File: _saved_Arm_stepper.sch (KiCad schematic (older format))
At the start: 126 parts, among them IC1 L6208D, IC2 L6208D, J1 12V_CONN, J10 ENCODER1, J11 ENCODER2, J2 M1_CONN, J3 M1_CONN, J4 Conn_01x06_Male, J5 I2C_CONN, J8 Conn_01x04_Female, J9 USB_B_Mini, M2 Fan, Q2 2N2219, SW1 SW_Push_Dual, SW2 endstop4, SW3 endstop1, SW4 endstop3, SW5 endstop2, U1 ISO1050-00_isolation, U2 USBLC6-2SC6, U3 STM32F446RETx, U4 LM1117-3.3, U5 LM1117-5, Y1 8Mhz

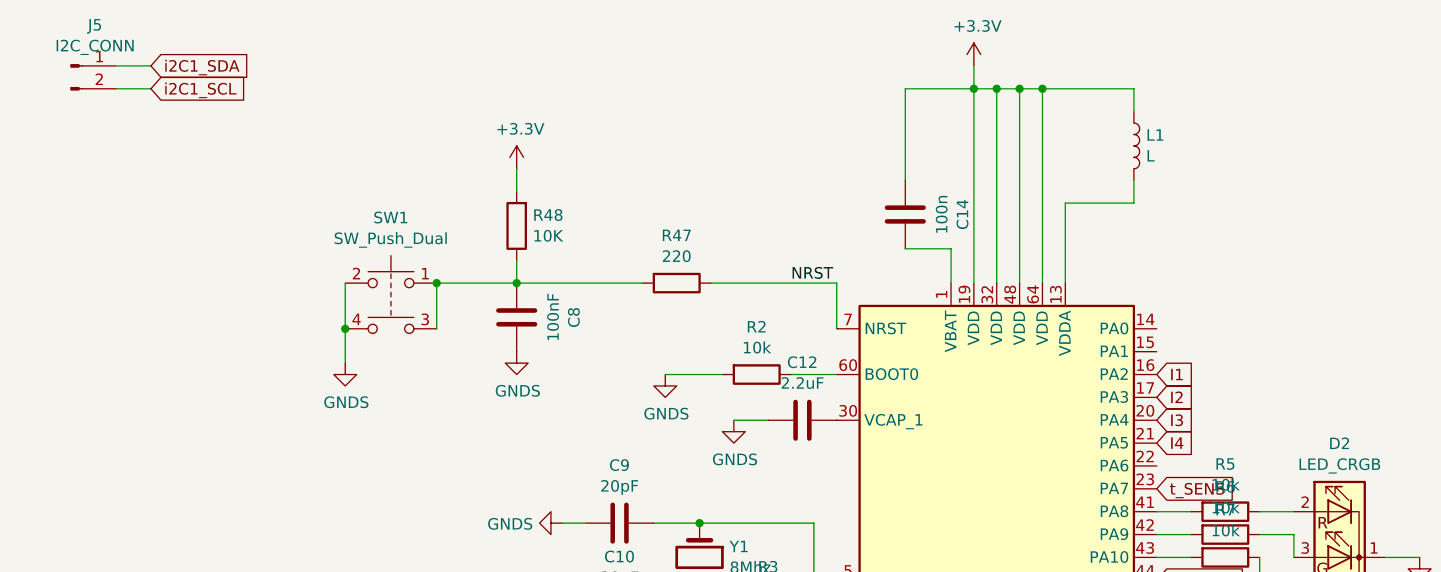
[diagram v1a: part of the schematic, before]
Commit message: finish4
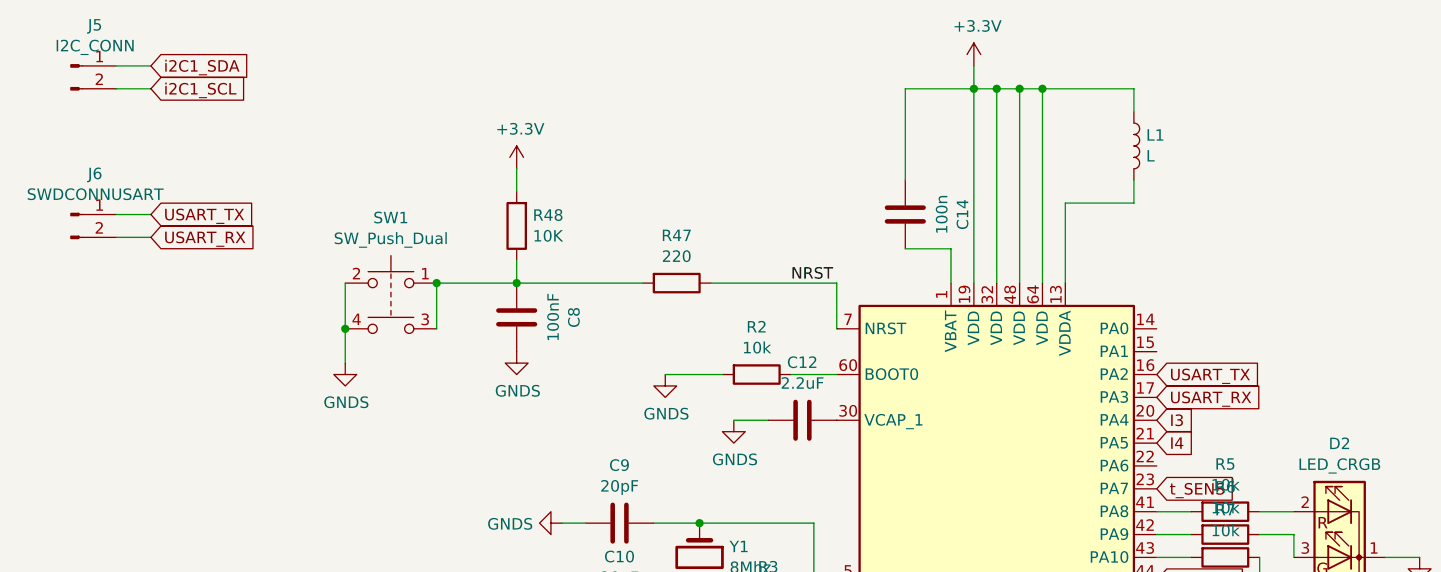
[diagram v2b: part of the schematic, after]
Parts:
- added J6: SWDCONNUSART, TerminalBlock_Phoenix:TerminalBlock_Phoenix_MPT-0,5-4-2.54_1x04_P2.54mm_Horizontal, symbol Connector:Conn_01x02_Male
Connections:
- net I1 renamed USART_TX
- net USART_TX: now also J6.1 (Pin_1)
- net I2 renamed USART_RX
- net USART_RX: now also J6.2 (Pin_2)
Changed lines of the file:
@@
 CAN_TX
 Text GLabel 5400 2900 2    50   Input ~ 0
-I1
+USART_TX
 Text GLabel 5400 3000 2    50   Input ~ 0
-I2
+USART_RX
 Text GLabel 5400 3400 2    50   Input ~ 0
 t_SENS
@@
 	1    0    0    -1
 $EndComp
+Wire Wire Line
+	850  2300 1000 2300
+Wire Wire Line
+	850  2200 1000 2200
+$Comp
+L Connector:Conn_01x02_Male J6
+U 1 1 5C859CCF
+P 650 2200
+F 0 "J6" H 756 2378 50  0000 C CNN
+F 1 "SWDCONNUSART" H 756 2287 50  0000 C CNN
+F 2 "TerminalBlock_Phoenix:TerminalBlock_Phoenix_MPT-0,5-4-2.54_1x04_P2.54mm_Horizontal" H 650 2200 50  0001 C CNN
+F 3 "~" H 650 2200 50  0001 C CNN
+	1    650  2200
+	1    0    0    -1
+$EndComp
+Text GLabel 1000 2200 2    50   Input ~ 0
+USART_TX
+Text GLabel 1000 2300 2    50   Input ~ 0
+USART_RX
 $EndSCHEMATC
